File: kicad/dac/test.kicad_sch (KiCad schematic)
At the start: 20 parts, among them U1 PCM2704/4C/5/5C, U1 PCM510xA, Y1 12MHz±0.05%

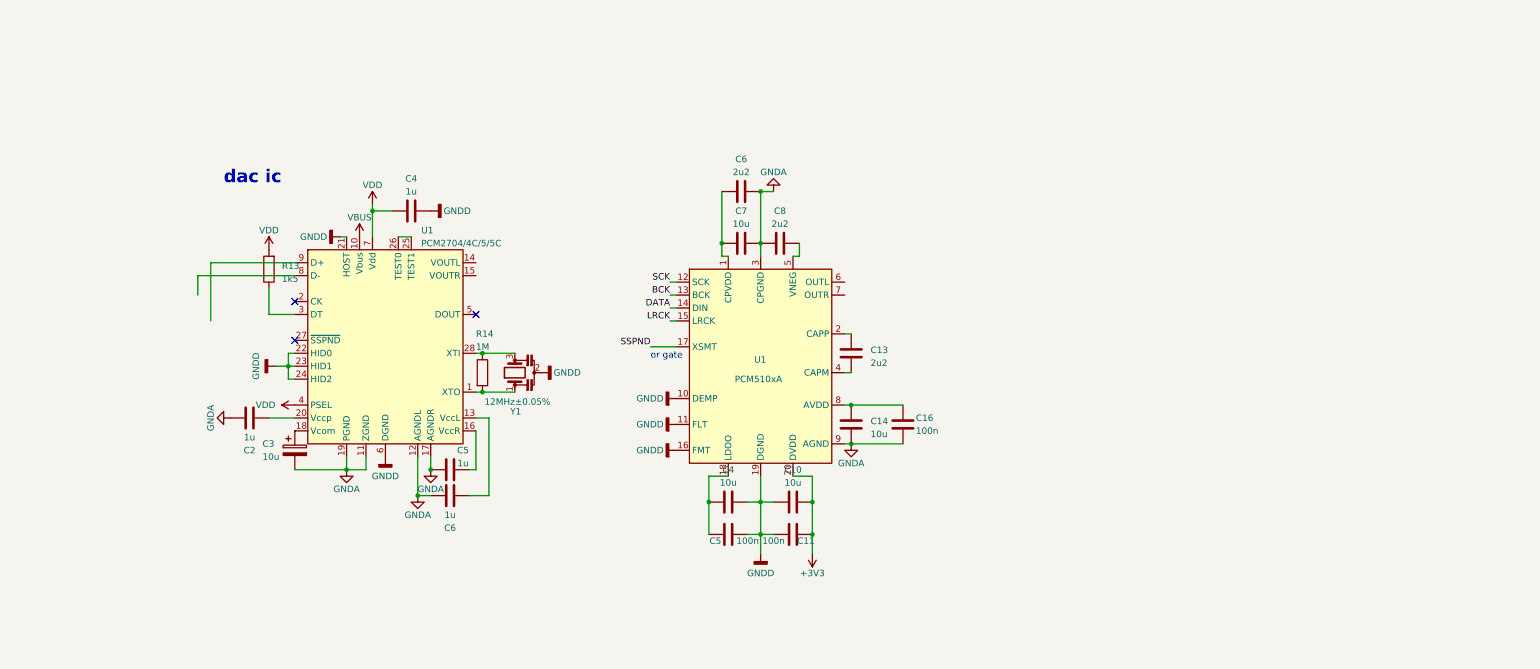
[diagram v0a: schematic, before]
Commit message: commit
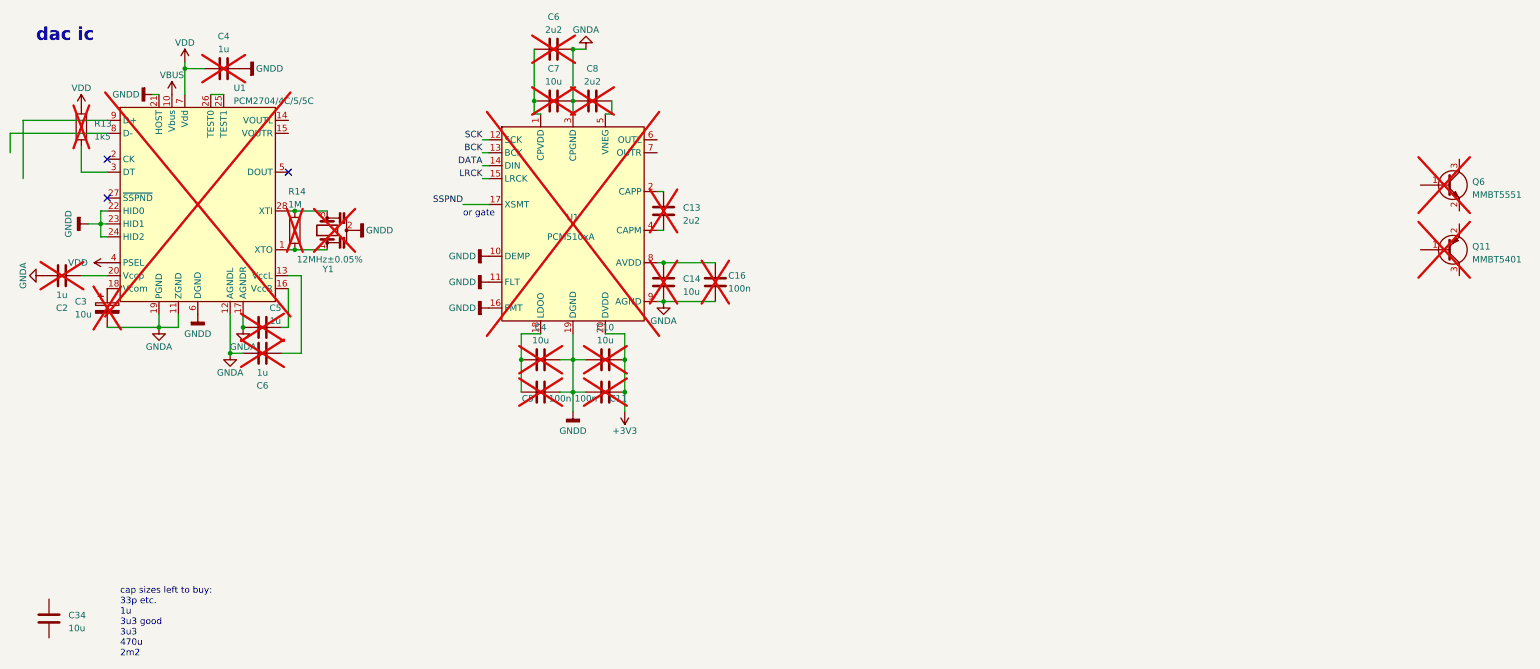
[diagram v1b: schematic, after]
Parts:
- added C34: 10u, symbol Device:C
- added Q11: MMBT5401, Package_TO_SOT_SMD:SOT-23-3, symbol Device:Q_PNP_BEC
- added Q6: MMBT5551, Package_TO_SOT_SMD:SOT-23-3, symbol Device:Q_NPN_BEC
- C10, C11, C13, C14, C16, C2, C3, C4, C5, C6, C7, C8, R13, R14, U1, Y1: now not fitted
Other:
- note added: "cap sizes left to buy: 33p etc. 1u 3u3 good 3u3 470u 2m2"
